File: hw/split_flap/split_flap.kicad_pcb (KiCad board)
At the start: 2 copper layers, 104.5 x 98.3 mm, 38 parts, among them J1 Conn_01x02, J10 Conn_01x05, J11 Conn_01x05, J12 Conn_01x05, J13 Conn_01x05, J14 Conn_01x05, J15 Conn_01x05, J16 Conn_01x05, J19 POWER, J2 Conn_01x02, J3 Conn_01x02, J4 Conn_01x02, J5 Conn_01x02, J6 Conn_01x02, J7 Conn_01x02, J8 Conn_01x02, J9 Conn_01x05, SW1 SW_RESET, U1 PCF8574, U10 ULN2803A, U2 NodeMCU_1.0_(ESP-12E), U3 PCF8574, U4 ULN2803A, U5 PCF8574, U6 ULN2803A, U7 PCF8574, U8 ULN2803A, U9 PCF8574

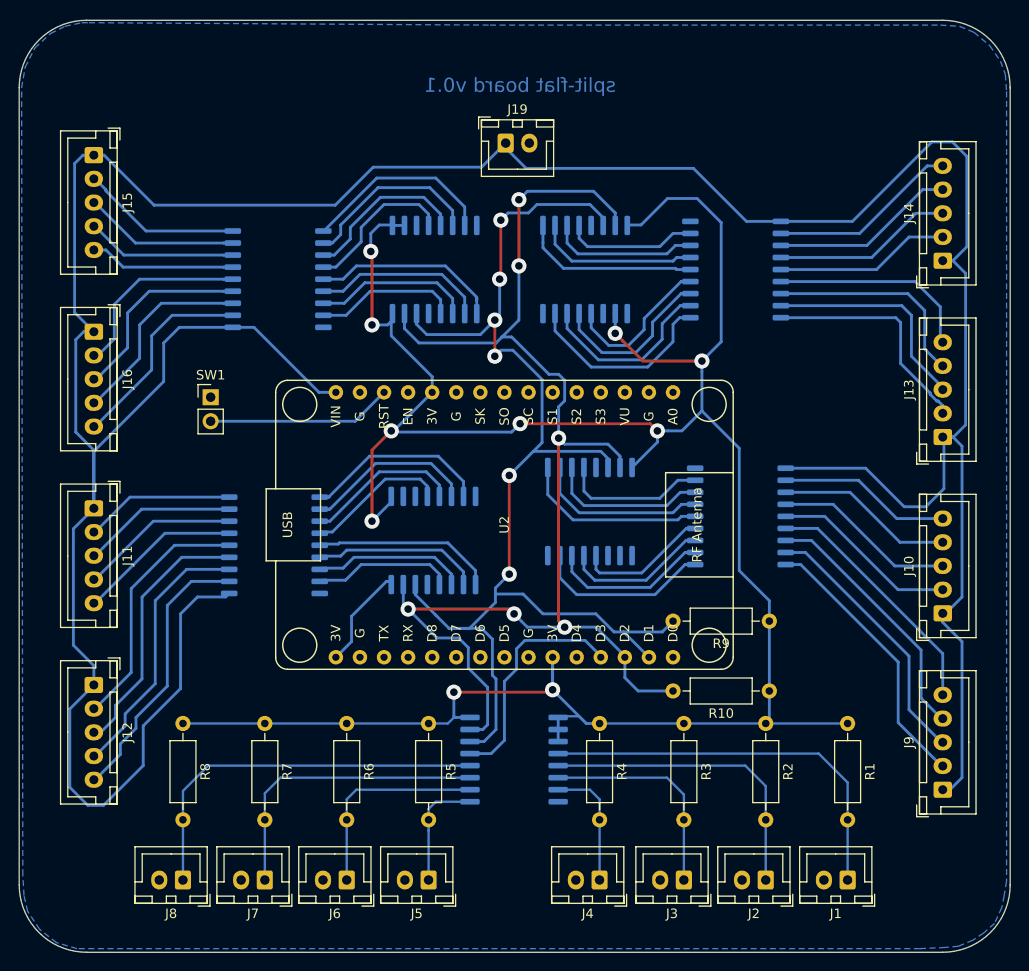
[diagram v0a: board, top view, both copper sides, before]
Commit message: hw: Supercharge PCB !
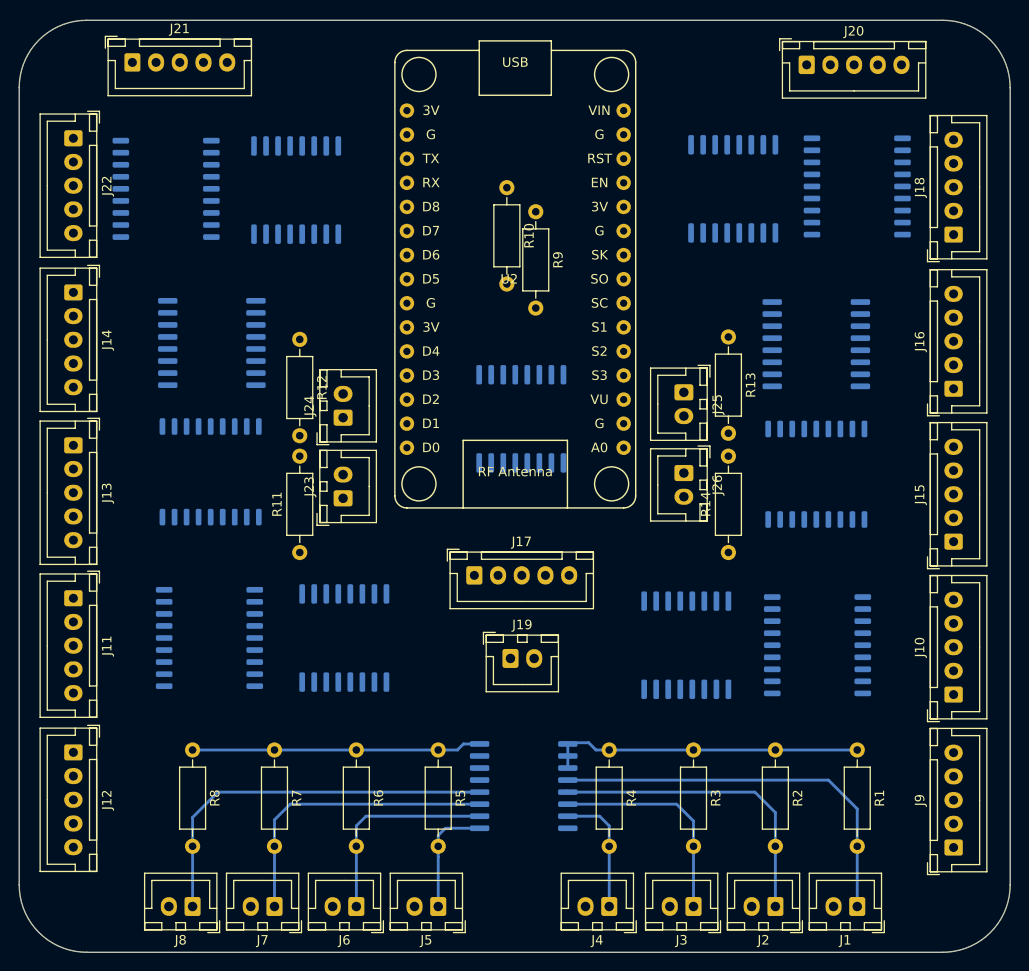
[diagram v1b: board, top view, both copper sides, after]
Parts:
- removed SW1: SW_RESET, Connector_PinHeader_2.54mm:PinHeader_1x02_P2.54mm_Vertical
- added J17: Conn_01x05, Connector_JST:JST_XH_B5B-XH-A_1x05_P2.50mm_Vertical, F.Cu at (144.4, 99.7)
- added J18: Conn_01x05, Connector_JST:JST_XH_B5B-XH-A_1x05_P2.50mm_Vertical, F.Cu at (194.9, 63.8)
- added J20: Conn_01x05, Connector_JST:JST_XH_B5B-XH-A_1x05_P2.50mm_Vertical, F.Cu at (179.5, 45.8)
- added J21: Conn_01x05, Connector_JST:JST_XH_B5B-XH-A_1x05_P2.50mm_Vertical, F.Cu at (108.3, 45.6)
- added J22: Conn_01x05, Connector_JST:JST_XH_B5B-XH-A_1x05_P2.50mm_Vertical, F.Cu at (102.1, 53.6)
- added J23: Conn_01x02, Connector_JST:JST_XH_B2B-XH-A_1x02_P2.50mm_Vertical, F.Cu at (130.6, 91.6)
- added J24: Conn_01x02, Connector_JST:JST_XH_B2B-XH-A_1x02_P2.50mm_Vertical, F.Cu at (130.6, 83.1)
- added J25: Conn_01x02, Connector_JST:JST_XH_B2B-XH-A_1x02_P2.50mm_Vertical, F.Cu at (166.5, 80.4)
- added J26: Conn_01x02, Connector_JST:JST_XH_B2B-XH-A_1x02_P2.50mm_Vertical, F.Cu at (166.5, 88.9)
- added R11: R, Resistor_THT:R_Axial_DIN0207_L6.3mm_D2.5mm_P10.16mm_Horizontal, F.Cu at (126.0, 97.3)
- added R12: R, Resistor_THT:R_Axial_DIN0207_L6.3mm_D2.5mm_P10.16mm_Horizontal, F.Cu at (126.0, 74.8)
- added R13: R, Resistor_THT:R_Axial_DIN0207_L6.3mm_D2.5mm_P10.16mm_Horizontal, F.Cu at (171.2, 74.5)
- added R14: R, Resistor_THT:R_Axial_DIN0207_L6.3mm_D2.5mm_P10.16mm_Horizontal, F.Cu at (171.2, 97.3)
- added U11: PCF8574, Package_SO:SOIC-16W_7.5x10.3mm_P1.27mm, B.Cu at (171.7, 58.9)
- added U12: ULN2803A, Package_SO:SOP-18_7x12.5mm_P1.27mm, B.Cu at (184.8, 58.7)
- added U13: PCF8574, Package_SO:SOIC-16W_7.5x10.3mm_P1.27mm, B.Cu at (125.6, 59.1)
- added U14: ULN2803A, Package_SO:SOP-18_7x12.5mm_P1.27mm, B.Cu at (111.9, 58.9)
- added U15: PCF8574, Package_SO:SOIC-16W_7.5x10.3mm_P1.27mm, B.Cu at (149.4, 83.2)
- U2: footprint ESP:NodeMCU1.0(12-E) -> ESP:ESP12F-Devkit-V3
- moved J15 99.4 mm to (194.9, 96.1), turned to 90 degrees
- moved J14 91.8 mm to (102.1, 69.8), turned to 270 degrees
- moved J13 91.7 mm to (102.1, 86.0), turned to 270 degrees
- moved J16 90.9 mm to (194.9, 80.0), turned to 90 degrees
- moved U10 60.4 mm to (180.5, 89.0), turned to 270 degrees
- moved R10 59.9 mm to (147.8, 58.8), turned to 270 degrees
- moved U8 59.3 mm to (116.6, 88.8), turned to 270 degrees
- moved J19 54.4 mm to (148.2, 108.5)
- moved R9 49.7 mm to (150.9, 61.3), turned to 270 degrees
- moved U9 41.0 mm to (180.5, 75.3), turned to 180 degrees
- moved U7 40.1 mm to (116.7, 75.2), turned to 180 degrees
- moved U2 27.2 mm to (148.7, 67.2), turned to 180 degrees
- moved U3 17.4 mm to (166.8, 107.1), turned to 270 degrees
- moved U4 15.8 mm to (180.6, 107.1)
- moved U5 13.9 mm to (130.7, 106.3), turned to 90 degrees
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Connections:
- U10 pad 1: Net-(U10-Pad1) -> /sheet5DE57FF1/L5
- U10 pad 11: Net-(J16-Pad5) -> Net-(J16-Pad2)
- U10 pad 12: Net-(J16-Pad4) -> Net-(J16-Pad3)
- U10 pad 13: Net-(J16-Pad3) -> Net-(J16-Pad4)
- U10 pad 14: Net-(J16-Pad2) -> Net-(J16-Pad5)
- U10 pad 2: Net-(U10-Pad2) -> /sheet5DE57FF1/L6
- U10 pad 3: Net-(U10-Pad3) -> /sheet5DE57FF1/L7
- U10 pad 4: Net-(U10-Pad4) -> /sheet5DE57FF1/L8
- U10 pad 5: Net-(U10-Pad5) -> /sheet5DE57FF1/L1
- U10 pad 6: Net-(U10-Pad6) -> /sheet5DE57FF1/L2
- U10 pad 7: Net-(U10-Pad7) -> /sheet5DE57FF1/L3
- U10 pad 8: Net-(U10-Pad8) -> /sheet5DE57FF1/L4
- U2 pad 13: Net-(SW1-Pad2) -> (no net)
- U2 pad 14: GND -> (no net)
- U2 pad 27: /INT -> (no net)
- U2 pad 30: (no net) -> /INT
- U3 pad 10: Net-(U3-Pad10) -> /SheetMotor1/L6
- U3 pad 11: Net-(U3-Pad11) -> /SheetMotor1/L7
- U3 pad 12: Net-(U3-Pad12) -> /SheetMotor1/L8
- U3 pad 4: Net-(U3-Pad4) -> /SheetMotor1/L1
- U3 pad 5: Net-(U3-Pad5) -> /SheetMotor1/L2
- U3 pad 6: Net-(U3-Pad6) -> /SheetMotor1/L3
- U3 pad 7: Net-(U3-Pad7) -> /SheetMotor1/L4
- U3 pad 9: Net-(U3-Pad9) -> /SheetMotor1/L5
- U4 pad 1: Net-(U3-Pad7) -> /SheetMotor1/L5
- U4 pad 2: Net-(U3-Pad6) -> /SheetMotor1/L6
- U4 pad 3: Net-(U3-Pad5) -> /SheetMotor1/L7
- U4 pad 4: Net-(U3-Pad4) -> /SheetMotor1/L8
- U4 pad 5: Net-(U3-Pad9) -> /SheetMotor1/L1
- U4 pad 6: Net-(U3-Pad10) -> /SheetMotor1/L2
- U4 pad 7: Net-(U3-Pad11) -> /SheetMotor1/L3
- U4 pad 8: Net-(U3-Pad12) -> /SheetMotor1/L4
- U5 pad 10: Net-(U5-Pad10) -> /sheetMotor2/L6
- U5 pad 11: Net-(U5-Pad11) -> /sheetMotor2/L7
- U5 pad 12: Net-(U5-Pad12) -> /sheetMotor2/L8
- U5 pad 4: Net-(U5-Pad4) -> /sheetMotor2/L1
- U5 pad 5: Net-(U5-Pad5) -> /sheetMotor2/L2
- U5 pad 6: Net-(U5-Pad6) -> /sheetMotor2/L3
- U5 pad 7: Net-(U5-Pad7) -> /sheetMotor2/L4
- U5 pad 9: Net-(U5-Pad9) -> /sheetMotor2/L5
- U6 pad 1: Net-(U5-Pad7) -> /sheetMotor2/L5
- U6 pad 2: Net-(U5-Pad6) -> /sheetMotor2/L6
- U6 pad 3: Net-(U5-Pad5) -> /sheetMotor2/L7
- U6 pad 4: Net-(U5-Pad4) -> /sheetMotor2/L8
- U6 pad 5: Net-(U5-Pad9) -> /sheetMotor2/L1
- U6 pad 6: Net-(U5-Pad10) -> /sheetMotor2/L2
- U6 pad 7: Net-(U5-Pad11) -> /sheetMotor2/L3
- U6 pad 8: Net-(U5-Pad12) -> /sheetMotor2/L4
- U7 pad 10: Net-(U7-Pad10) -> /Sheet5DE1D348/L6
- U7 pad 11: Net-(U7-Pad11) -> /Sheet5DE1D348/L7
- U7 pad 12: Net-(U7-Pad12) -> /Sheet5DE1D348/L8
- U7 pad 4: Net-(U7-Pad4) -> /Sheet5DE1D348/L1
- U7 pad 5: Net-(U7-Pad5) -> /Sheet5DE1D348/L2
- U7 pad 6: Net-(U7-Pad6) -> /Sheet5DE1D348/L3
- U7 pad 7: Net-(U7-Pad7) -> /Sheet5DE1D348/L4
- U7 pad 9: Net-(U7-Pad9) -> /Sheet5DE1D348/L5
- U8 pad 1: Net-(U7-Pad7) -> /Sheet5DE1D348/L5
- U8 pad 11: Net-(J14-Pad5) -> Net-(J14-Pad2)
- U8 pad 12: Net-(J14-Pad4) -> Net-(J14-Pad3)
- U8 pad 13: Net-(J14-Pad3) -> Net-(J14-Pad4)
- U8 pad 14: Net-(J14-Pad2) -> Net-(J14-Pad5)
- U8 pad 2: Net-(U7-Pad6) -> /Sheet5DE1D348/L6
- U8 pad 3: Net-(U7-Pad5) -> /Sheet5DE1D348/L7
- U8 pad 4: Net-(U7-Pad4) -> /Sheet5DE1D348/L8
- U8 pad 5: Net-(U7-Pad9) -> /Sheet5DE1D348/L1
- U8 pad 6: Net-(U7-Pad10) -> /Sheet5DE1D348/L2
- U8 pad 7: Net-(U7-Pad11) -> /Sheet5DE1D348/L3
- U8 pad 8: Net-(U7-Pad12) -> /Sheet5DE1D348/L4
- U9 pad 10: Net-(U10-Pad6) -> /sheet5DE57FF1/L6
- U9 pad 11: Net-(U10-Pad7) -> /sheet5DE57FF1/L7
- U9 pad 12: Net-(U10-Pad8) -> /sheet5DE57FF1/L8
- U9 pad 4: Net-(U10-Pad4) -> /sheet5DE57FF1/L1
- U9 pad 5: Net-(U10-Pad3) -> /sheet5DE57FF1/L2
- U9 pad 6: Net-(U10-Pad2) -> /sheet5DE57FF1/L3
- U9 pad 7: Net-(U10-Pad1) -> /sheet5DE57FF1/L4
- U9 pad 9: Net-(U10-Pad5) -> /sheet5DE57FF1/L5
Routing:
- net +5V: track 355.0 -> 0.00 mm
- net +3V3: track 265.6 -> 64.5 mm, vias 10 -> 0
- net /SDA: track 138.9 -> 0.00 mm, vias 6 -> 0
- net /SCL: track 133.4 -> 0.00 mm, vias 6 -> 0
- net Net-(J12-Pad5): track 29.2 -> 0.00 mm
- net Net-(J9-Pad2): track 29.1 -> 0.00 mm
- net Net-(J12-Pad4): track 28.3 -> 0.00 mm
- net Net-(J9-Pad3): track 28.2 -> 0.00 mm
- net Net-(J12-Pad3): track 27.7 -> 0.00 mm
- net Net-(J9-Pad4): track 27.3 -> 0.00 mm
- net Net-(J12-Pad2): track 26.6 -> 0.00 mm
- net Net-(J9-Pad5): track 26.4 -> 0.00 mm
- net /INT: track 24.5 -> 0.00 mm
- net Net-(J13-Pad2): track 24.3 -> 0.00 mm
- net Net-(J13-Pad3): track 23.4 -> 0.00 mm
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- removed copper zone on B.Cu, net GND
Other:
- board text removed: "split-flat board v0.1"
